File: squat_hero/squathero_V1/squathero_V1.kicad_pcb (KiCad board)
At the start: 2 copper layers, 36.5 x 31.5 mm, 6 parts, among them U2 AMS1117

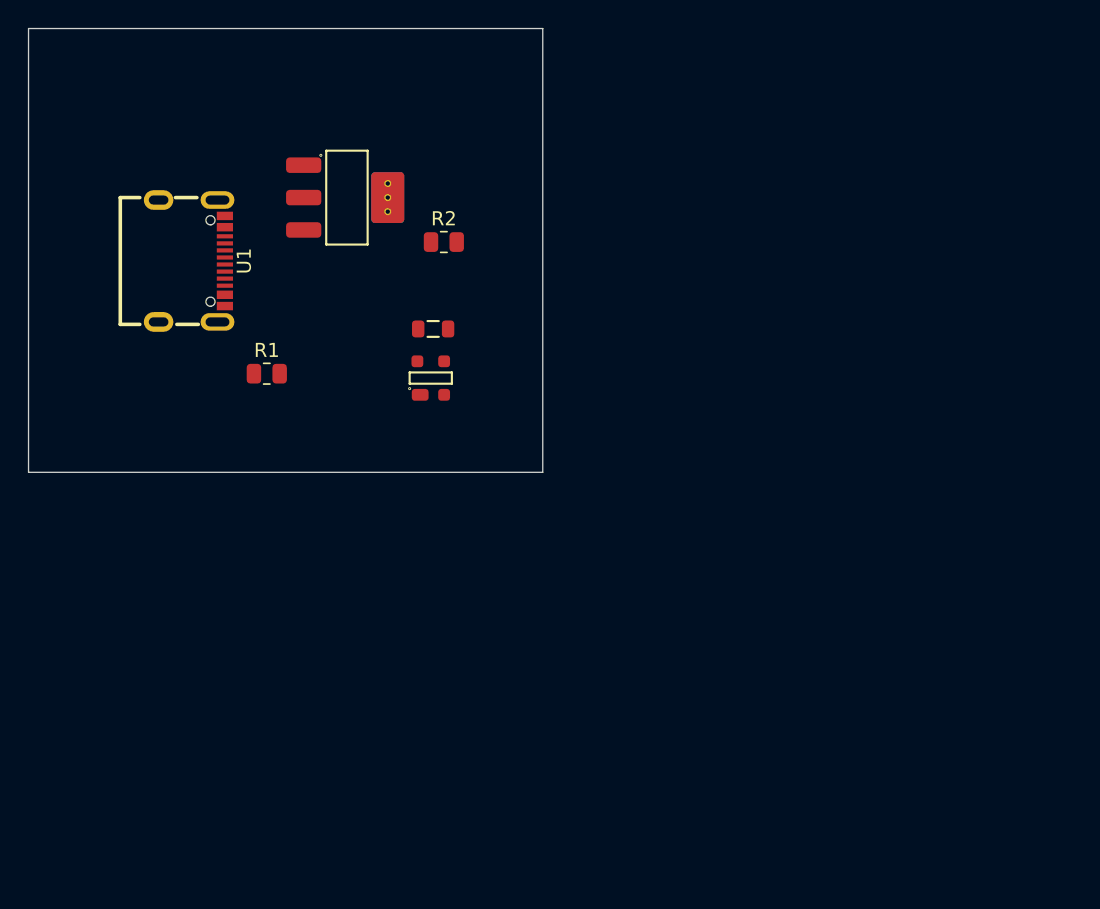
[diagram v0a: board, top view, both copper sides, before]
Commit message: V1 squat hero
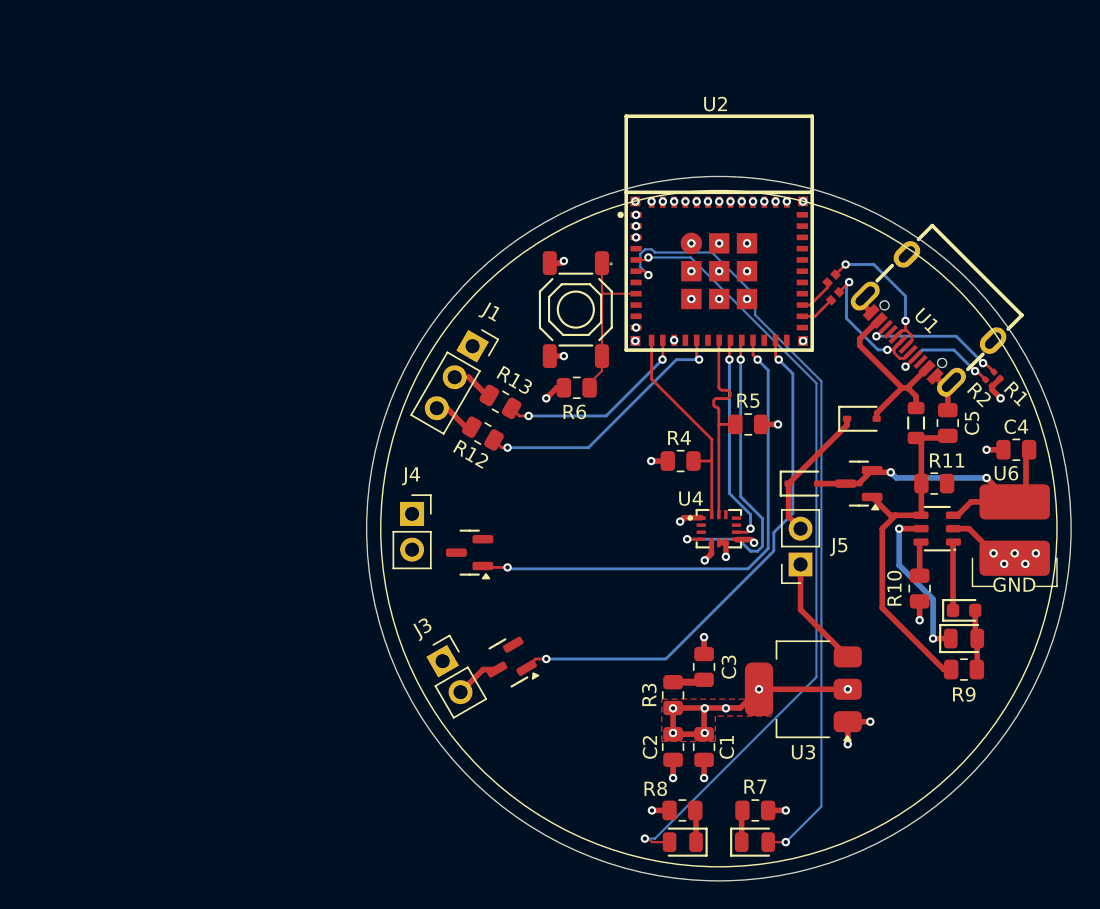
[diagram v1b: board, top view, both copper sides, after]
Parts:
- removed FB1: ~, PCM_JLCPCB:FB_0805
- added C1: 1uF, Resistor_SMD:R_0805_2012Metric, F.Cu at (148.9, 115.5)
- added C2: 10nF, Resistor_SMD:R_0805_2012Metric, F.Cu at (146.8, 115.5)
- added C3: 1uF, Resistor_SMD:R_0805_2012Metric, F.Cu at (148.9, 109.8)
- added C4: 1uF, Resistor_SMD:R_0805_2012Metric, F.Cu at (171.1, 94.4)
- added C5: 1uF, Resistor_SMD:R_0805_2012Metric, F.Cu at (166.2, 92.5)
- added D2: Yellow, PCM_JLCPCB:D_0805, F.Cu at (147.4, 122.2)
- added D3: Green, PCM_JLCPCB:D_0805, F.Cu at (167.4, 107.8)
- added D4: Red, PCM_JLCPCB:D_0603, F.Cu at (167.4, 105.8)
- added D5: 1N5819WS, PCM_JLCPCB:D_SOD-323, F.Cu at (160.2, 92.2)
- added D6: 1N5819WS, PCM_JLCPCB:D_SOD-323, F.Cu at (156.0, 96.8)
- added D7: H3V3L10B, PCM_JLCPCB:D_DFN1006-2L, F.Cu at (158.0, 82.2)
- added D8: H3V3L10B, PCM_JLCPCB:D_DFN1006-2L, F.Cu at (158.2, 83.5)
- added FB2: ~, PCM_JLCPCB:FB_0805, F.Cu at (164.0, 92.5)
- added J1: Conn_01x03, Connector_PinSocket_2.54mm:PinSocket_1x03_P2.54mm_Vertical, F.Cu at (132.5, 87.1)
- added J3: Conn_01x02, Connector_PinSocket_2.54mm:PinSocket_1x02_P2.54mm_Vertical, F.Cu at (130.4, 109.4)
- added J4: Conn_01x02, Connector_PinSocket_2.54mm:PinSocket_1x02_P2.54mm_Vertical, F.Cu at (128.2, 99.0)
- added J5: Conn_01x02, Connector_PinSocket_2.54mm:PinSocket_1x02_P2.54mm_Vertical, F.Cu at (155.8, 102.5)
- added Q1: HL2307, PCM_JLCPCB:Q_SOT-23, F.Cu at (135.1, 109.5)
- added Q2: HL2307, PCM_JLCPCB:Q_SOT-23, F.Cu at (132.3, 101.7)
- added Q3: HL2307, PCM_JLCPCB:Q_SOT-23, F.Cu at (159.9, 96.8)
- added R10: 2.5k, Resistor_SMD:R_0805_2012Metric, F.Cu at (164.2, 104.2)
- added R11: 10k, Resistor_SMD:R_0805_2012Metric, F.Cu at (165.3, 96.8)
- added R12: 330, Resistor_SMD:R_0805_2012Metric, F.Cu at (133.2, 93.2)
- added R13: 330, Resistor_SMD:R_0805_2012Metric, F.Cu at (134.5, 91.0)
- added R3: 10k, Resistor_SMD:R_0805_2012Metric, F.Cu at (146.8, 111.8)
- added R4: 4.7k, Resistor_SMD:R_0805_2012Metric, F.Cu at (147.3, 95.2)
- added R5: 4.7k, Resistor_SMD:R_0805_2012Metric, F.Cu at (152.1, 92.6)
- added R6: 10k, Resistor_SMD:R_0805_2012Metric, F.Cu at (139.9, 90.0)
- added R7: 50, Resistor_SMD:R_0805_2012Metric, F.Cu at (152.6, 120.0)
- added R8: 50, Resistor_SMD:R_0805_2012Metric, F.Cu at (147.4, 120.0)
- added R9: 1k, Resistor_SMD:R_0805_2012Metric, F.Cu at (167.4, 110.0)
- added S1: Tactile Button, 160gf, PCM_JLCPCB:SW-SMD_4P-L5.1-W5.1-P3.70-LS6.5-TL-2, F.Cu at (139.8, 84.5)
- added U3: AMS1117-3.3, Package_TO_SOT_SMD:SOT-223-3_TabPin2, F.Cu at (156.0, 111.4)
- added U4: ~, imu:LGA-14_L3.0-W2.5-P0.50-TL_QMI8658A, F.Cu at (150.0, 100.0)
- added U5: TP4057, PCM_JLCPCB:SOT-23-6_L2.9-W1.6-P0.95-LS2.8-BL, F.Cu at (165.5, 100.0)
- added U6: ~, batt_conn:Untitled, F.Cu at (171.0, 100.1)
- D1: value H5VUT1B -> White; footprint PCM_JLCPCB:SOT-143-4_L2.9-W1.3-P1.90-LS2.4-BL-1 -> PCM_JLCPCB:D_0805
- R1, R2: footprint Resistor_SMD:R_0805_2012Metric -> Resistor_SMD:R_0201_0603Metric
- U1: footprint JLCPCB_USB-C:USB-SMD_TYPE-C16PIN-1 -> JLCPCB_USB_FOOTPRINT:USB-SMD_TYPE-C16PIN-1
- U2: value AMS1117 -> ~; footprint PCM_JLCPCB:SOT-223-3_L6.5-W3.4-P2.30-LS7.0-BR -> esp_32:WIFIM-SMD_ESP32-C3-MINI-1
- moved U1 52.3 mm to (164.7, 85.3), turned to 135 degrees
- moved R1 51.8 mm to (169.8, 89.1), turned to -45 degrees
- moved D1 40.2 mm to (152.6, 122.2)
- moved R2 39.9 mm to (169.2, 89.7), turned to -45 degrees
- moved U2 27.0 mm to (150.0, 81.7), turned to 0 degrees
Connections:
- D1 pad 1: /USB_D+ -> Net-(D1-Pad1)
- D1 pad 2: /USB_D- -> /DEBUG_LED1
- U2 pad 2: REG_3.3V -> GND
- U2 pad 3: /+5V -> /+3.3V
- U2 pad 4: REG_3.3V -> unconnected-(U2-NC-Pad4)
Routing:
- net /DEBUG_LED2: track 0.00 -> 56.2 mm, vias 0 -> 2
- net /DEBUG_LED1: track 0.00 -> 55.4 mm, vias 0 -> 2
- net /+5V: track 0.00 -> 39.3 mm
- net /PWM_1: track 0.00 -> 37.0 mm, vias 0 -> 2
- net /PWM_2: track 0.00 -> 36.2 mm, vias 0 -> 2
- net GND: track 0.00 -> 27.4 mm, vias 0 -> 49
- net /+3.3V: track 0.00 -> 25.6 mm, vias 0 -> 13
- net /BATT+: track 0.00 -> 24.2 mm, vias 0 -> 2
- net /I2C_INT1: track 0.00 -> 22.1 mm, vias 0 -> 2
- net /GPI0_10: track 0.00 -> 18.8 mm, vias 0 -> 2
- net /raw_power: track 0.00 -> 18.0 mm
- net /I2C_SCL_1: track 0.00 -> 15.4 mm
- net /I2C_SDA_1: track 0.00 -> 15.3 mm
- net /I2C_INT2: track 0.00 -> 15.1 mm, vias 0 -> 2
- net /GPI0_1: track 0.00 -> 14.0 mm, vias 0 -> 2
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- added copper zone on F.Cu, net /+3.3V
- added copper zone on In2.Cu, net /+3.3V
- added copper zone on In1.Cu, net GND
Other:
- board size 36.5 x 31.5 mm -> 50 x 50 mm
- copper layers 2 -> 4
